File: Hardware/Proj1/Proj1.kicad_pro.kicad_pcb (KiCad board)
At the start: 2 copper layers, 19 x 23 mm, 6 parts, among them J1 Conn_01x02, SW1 SW_Push

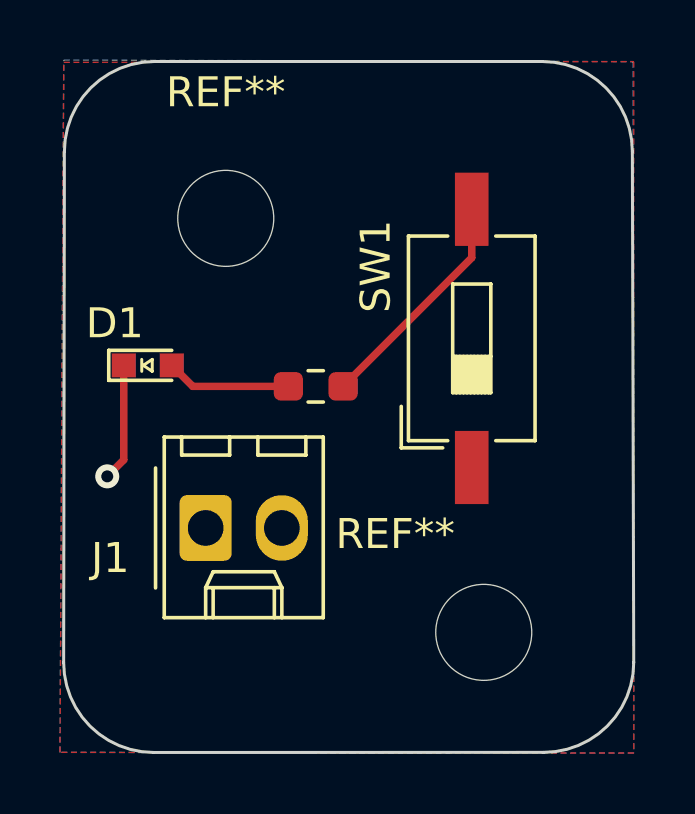
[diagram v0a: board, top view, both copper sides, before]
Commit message: Please review my updated PCB LED and my Firware Heartbeat Project.
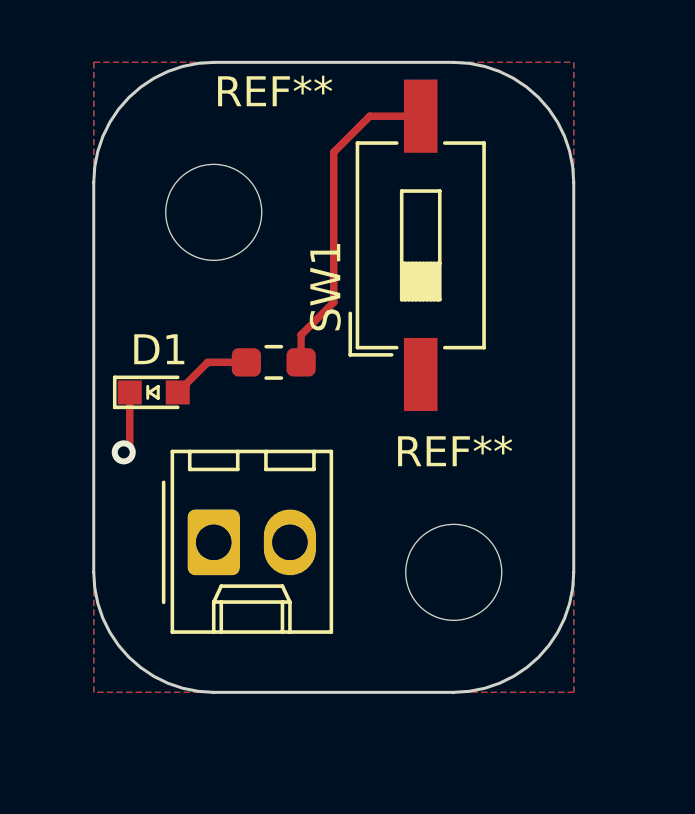
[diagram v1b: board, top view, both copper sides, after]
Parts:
- moved SW1 3.54 mm to (163.9, 120.1)
- moved REF** 2.24 mm to (165.0, 131.0)
- moved R1 1.61 mm to (159.0, 124.0)
- moved D1 0.92 mm to (155.0, 125.0)
- moved J1 0.55 mm to (157.0, 130.0)
- moved REF** 0.45 mm to (157.0, 119.0)
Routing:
- net Net-(R1-Pad1): track 7.68 -> 10.8 mm
- net GND: track 3.93 -> 2.08 mm
- net Net-(D1-A): track 4.18 -> 2.70 mm
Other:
- board size 19 x 23 mm -> 16 x 21 mm
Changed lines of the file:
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@@
 	(footprint "Button_Switch_SMD:SW_DIP_SPSTx01_Slide_6.7x4.1mm_W8.61mm_P2.54mm_LowProfile"
 		(layer "F.Cu")
-		(at 165.6 123.2 90)
+		(at 163.9 120.1 90)
 		(descr "SMD 1x-dip-switch SPST , Slide, row spacing 8.61 mm (338 mils), body size 6.7x4.1mm (see e.g. https://www.ctscorp.com/wp-content/uploads/219.pdf), SMD, LowProfile")
 		(tags "SMD DIP Switch SPST Slide 8.61mm 338mil SMD LowProfile")
 		(property "Reference" "SW1"
-			(at 2.4 -3.2 90)
+			(at -1.377 -3.1446 90)
 			(layer "F.SilkS")
 			(effects
@@
 			(at 0 3.11 90)
 			(layer "F.Fab")
+			(hide yes)
 			(effects
 				(font
@@
 		)
 		(fp_text user "${REFERENCE}"
-			(at 2.58 0 360)
+			(at 2.58 0 0)
 			(layer "F.Fab")
 			(effects
@@
 	(footprint "MountingHole:MountingHole_3.2mm_M3"
 		(layer "F.Cu")
-		(at 166 133)
+		(at 165 131)
 		(descr "Mounting Hole 3.2mm, no annular, M3")
 		(tags "mounting hole 3.2mm no annular m3")
 		(property "Reference" "REF**"
-			(at -2.95 -3.275 0)
+			(at 0 -4 0)
 			(layer "F.SilkS")
 			(effects
@@
 			(at -4.8 2.5 0)
 			(layer "F.Fab")
+			(hide yes)
 			(effects
 				(font
@@
 			(at 0 0 0)
 			(layer "F.Fab")
+			(hide yes)
 			(effects
 				(font
@@
 			(size 3.2 3.2)
 			(drill 3.2)
-			(layers "*.Cu" "*.Mask")
+			(layers "F&B.Cu" "*.Mask")
 		)
 	)
 	(footprint "MountingHole:MountingHole_3.2mm_M3"
 		(layer "F.Cu")
-		(at 157.4 119.2)
+		(at 157 119)
 		(descr "Mounting Hole 3.2mm, no annular, M3")
 		(tags "mounting hole 3.2mm no annular m3")
 		(property "Reference" "REF**"
-			(at 0 -4.2 0)
+			(at 2 -4 0)
 			(layer "F.SilkS")
 			(effects
@@
 		)
 		(property "Value" "M1"
-			(at 0.1 4.7 0)
-			(layer "F.Fab")
+			(at -8 0 0)
+			(layer "F.Fab")
+			(hide yes)
 			(effects
 				(font
@@
 		)
 		(fp_text user "${REFERENCE}"
-			(at 0 0 0)
-			(layer "F.Fab")
+			(at -5 1 0)
+			(layer "F.Fab")
+			(hide yes)
 			(effects
 				(font
@@
 			(size 3.2 3.2)
 			(drill 3.2)
-			(layers "*.Cu" "*.Mask")
+			(layers "F&B.Cu" "*.Mask")
 		)
 	)
 	(footprint "Connector_Molex:Molex_KK-254_AE-6410-02A_1x02_P2.54mm_Vertical"
 		(layer "F.Cu")
-		(at 156.73 129.52)
+		(at 157 130)
 		(descr "Molex KK-254 Interconnect System, old/engineering part number: AE-6410-02A example for new part number: 22-27-2021, 2 Pins (http://www.molex.com/pdm_docs/sd/022272021_sd.pdf), generated with kicad-footprint-generator")
 		(tags "connector Molex KK-254 vertical")
@@
 			(at -3.18 1.005 0)
 			(layer "F.SilkS")
+			(hide yes)
 			(effects
 				(font
@@
 			(at 1.27 4.08 0)
 			(layer "F.Fab")
+			(hide yes)
 			(effects
 				(font
@@
 		)
 		(fp_text user "${REFERENCE}"
-			(at 1.27 -2.22 0)
+			(at 1.1 -3.9 0)
 			(layer "F.Fab")
 			(effects
@@
 	(footprint "layout:LED_0603_Symbol_on_F.SilkS"
 		(layer "F.Cu")
-		(at 154.8 124.1)
+		(at 155 125)
 		(descr "LED 0603 smd package")
 		(tags "LED led 0603 SMD smd SMT smt smdled SMDLED smtled SMTLED")
 		(property "Reference" "D1"
-			(at -1.1 -1.4 0)
+			(at 0.1804 -1.4 0)
 			(layer "F.SilkS")
 			(effects
@@
 			(at 0 1.35 0)
 			(layer "F.Fab")
+			(hide yes)
 			(effects
 				(font
@@
 	(footprint "Resistor_SMD:R_0603_1608Metric_Pad0.98x0.95mm_HandSolder"
 		(layer "F.Cu")
-		(at 160.4 124.8 180)
+		(at 159 124 180)
 		(descr "Resistor SMD 0603 (1608 Metric), square (rectangular) end terminal, IPC_7351 nominal with elongated pad for handsoldering. (Body size source: IPC-SM-782 page 72, https://www.pcb-3d.com/wordpress/wp-content/uploads/ipc-sm-782a_amendment_1_and_2.pdf), generated with kicad-footprint-generator")
 		(tags "resistor handsolder")
 		(property "Reference" "R1"
-			(at -8.9 -16.57 360)
+			(at -8.9 -16.57 0)
 			(layer "F.SilkS")
 			(hide yes)
@@
 		)
 		(property "Value" "105"
-			(at 0 1.43 360)
-			(layer "F.Fab")
+			(at 0 1.43 0)
+			(layer "F.Fab")
+			(hide yes)
 			(effects
 				(font
@@
 		)
 		(property "Footprint" "Resistor_SMD:R_0603_1608Metric_Pad0.98x0.95mm_HandSolder"
-			(at 0 0 360)
+			(at 0 0 0)
 			(layer "F.Fab")
 			(hide yes)
@@
 		)
 		(property "Datasheet" ""
-			(at 0 0 360)
+			(at 0 0 0)
 			(layer "F.Fab")
 			(hide yes)
@@
 		)
 		(property "Description" "Resistor"
-			(at 0 0 360)
+			(at 0 0 0)
 			(layer "F.Fab")
 			(hide yes)
@@
 		)
 		(fp_text user "${REFERENCE}"
-			(at -0.0875 -1 360)
-			(layer "F.Fab")
-			(effects
-				(font
-					(size 0.4 0.4)
-					(thickness 0.06)
+			(at -0.3 1.3 0)
+			(layer "F.Fab")
+			(effects
+				(font
+					(size 1 1)
+					(thickness 0.15)
 				)
 			)
@@
 	)
 	(gr_line
-		(start 170.95368 116.97132)
-		(end 171 134)
+		(start 169 118)
+		(end 169 131)
 		(stroke
 			(width 0.1)
@@
 	)
 	(gr_arc
-		(start 152.02132 116.97132)
-		(mid 152.9 114.85)
-		(end 155.02132 113.97132)
+		(start 169 131)
+		(mid 167.828427 133.828427)
+		(end 165 135)
 		(stroke
 			(width 0.1)
@@
 	)
 	(gr_line
-		(start 155.02132 113.97132)
-		(end 167.95368 113.97132)
+		(start 153 131)
+		(end 153 118)
 		(stroke
 			(width 0.1)
@@
 	)
 	(gr_arc
-		(start 167.95368 113.97132)
-		(mid 170.075 114.85)
-		(end 170.95368 116.97132)
+		(start 165 114)
+		(mid 167.828427 115.171573)
+		(end 169 118)
 		(stroke
 			(width 0.1)
@@
 		(layer "Edge.Cuts")
 	)
-	(gr_arc
-		(start 154.99632 137.00368)
-		(mid 152.875 136.125)
-		(end 151.99632 134.00368)
+	(gr_line
+		(start 165 135)
+		(end 157 135)
 		(stroke
 			(width 0.1)
@@
 	)
 	(gr_line
-		(start 168 137)
-		(end 154.99632 137.00368)
+		(start 157 114)
+		(end 165 114)
 		(stroke
 			(width 0.1)
@@
 		(layer "Edge.Cuts")
 	)
-	(gr_line
-		(start 151.99632 134.00368)
-		(end 152.02132 116.97132)
+	(gr_arc
+		(start 153 118)
+		(mid 154.171573 115.171573)
+		(end 157 114)
 		(stroke
 			(width 0.1)
@@
 	)
 	(gr_arc
-		(start 171 134)
-		(mid 170.12132 136.12132)
-		(end 168 137)
+		(start 157 135)
+		(mid 154.171573 133.828427)
+		(end 153 131)
 		(stroke
 			(width 0.1)
@@
 		(layer "Dwgs.User")
 		(pts
-			(xy 152 140) (xy 171 140)
-		)
-		(height 0)
-		(gr_text "19.0000 mm"
-			(at 161.5 138.85 0)
+			(xy 165 131) (xy 165 119)
+		)
+		(height 7)
+		(gr_text "12.0000 mm"
+			(at 170.85 125 90)
 			(layer "Dwgs.User")
 			(effects
@@
 		(layer "Dwgs.User")
 		(pts
-			(xy 150 137) (xy 150 114)
-		)
-		(height -7)
-		(gr_text "23.0000 mm"
-			(at 141.85 125.5 90)
+			(xy 165 119) (xy 157 119)
+		)
+		(height 6)
+		(gr_text "8.0000 mm"
+			(at 161 111.85 0)
 			(layer "Dwgs.User")
 			(effects
@@
 		(layer "Dwgs.User")
 		(pts
-			(xy 166 133) (xy 157 133)
-		)
-		(height 21)
-		(gr_text "9.0000 mm"
-			(at 161.5 110.85 0)
+			(xy 153 139) (xy 169 139)
+		)
+		(height -1)
+		(gr_text "16.0000 mm"
+			(at 161 136.85 0)
 			(layer "Dwgs.User")
 			(effects
@@
 		(layer "Dwgs.User")
 		(pts
-			(xy 166 133) (xy 166 118)
-		)
-		(height 12)
-		(gr_text "15.0000 mm"
-			(at 176.85 125.5 90)
+			(xy 153 114) (xy 153 135)
+		)
+		(height 2)
+		(gr_text "21.0000 mm"
+			(at 149.85 124.5 90)
 			(layer "Dwgs.User")
 			(effects
@@
 	)
 	(segment
-		(start 156.3 124.8)
-		(end 155.6 124.1)
+		(start 156.8 124)
+		(end 155.8 125)
 		(width 0.25)
 		(layer "F.Cu")
@@
 	)
 	(segment
-		(start 159.4875 124.8)
-		(end 156.3 124.8)
+		(start 158.0875 124)
+		(end 156.8 124)
 		(width 0.25)
 		(layer "F.Cu")
@@
 	)
 	(segment
-		(start 154 127.25)
-		(end 153.45 127.8)
+		(start 154.2 126.8)
+		(end 154 127)
 		(width 0.25)
 		(layer "F.Cu")
@@
 	)
 	(segment
-		(start 154 124.1)
-		(end 154 127.25)
+		(start 154.2 125)
+		(end 154.2 126.8)
 		(width 0.25)
 		(layer "F.Cu")
@@
 	)
 	(via
-		(at 153.45 127.8)
+		(at 154 127)
 		(size 0.8)
 		(drill 0.4)
@@
 	)
 	(segment
-		(start 165.6 120.5125)
-		(end 161.3125 124.8)
+		(start 161 122)
+		(end 159.9125 123.0875)
 		(width 0.25)
 		(layer "F.Cu")
@@
 	)
 	(segment
-		(start 165.6 118.895)
-		(end 165.6 120.5125)
+		(start 161 117)
+		(end 161 122)
+		(width 0.25)
+		(layer "F.Cu")
+		(net 4)
+	)
+	(segment
+		(start 163.9 115.795)
+		(end 162.205 115.795)
+		(width 0.25)
+		(layer "F.Cu")
+		(net 4)
+	)
+	(segment
+		(start 162.205 115.795)
+		(end 161 117)
+		(width 0.25)
+		(layer "F.Cu")
+		(net 4)
+	)
+	(segment
+		(start 159.9125 123.0875)
+		(end 159.9125 124)
 		(width 0.25)
 		(layer "F.Cu")
@@
 		(polygon
 			(pts
-				(xy 152 114) (xy 171 113.975) (xy 171 137.025) (xy 151.875 137)
+				(xy 153 114) (xy 169 114) (xy 169 135) (xy 153 135)
 			)
 		)
@@
 		(polygon
 			(pts
-				(xy 152 113.925) (xy 170.975 113.975) (xy 171 137.025) (xy 151.875 137)
-			)
-		)
+				(xy 153 114) (xy 169 114) (xy 169 135) (xy 153 135)
+			)
+		)
